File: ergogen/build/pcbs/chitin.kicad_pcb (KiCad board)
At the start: 2 copper layers, 134 x 106.7 mm, 102 parts, among them J1 qwiik_jst

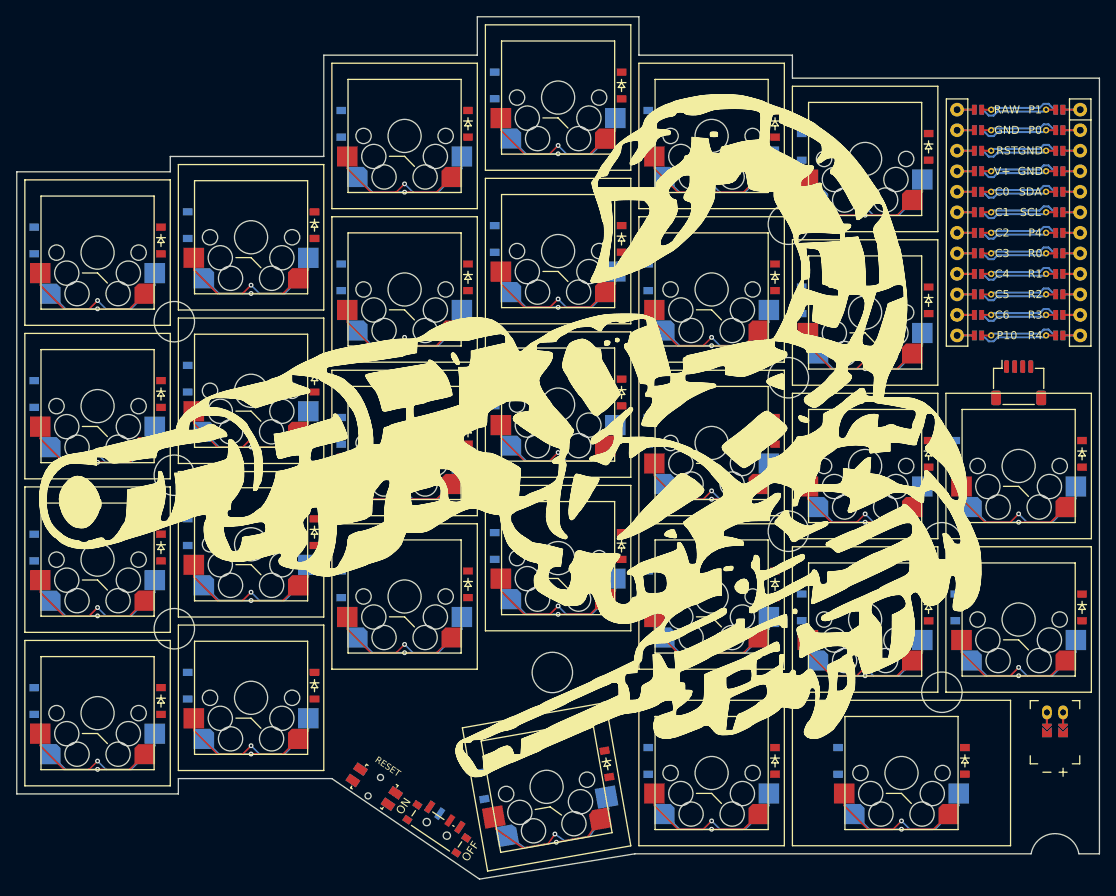
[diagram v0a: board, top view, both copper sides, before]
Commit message: Build
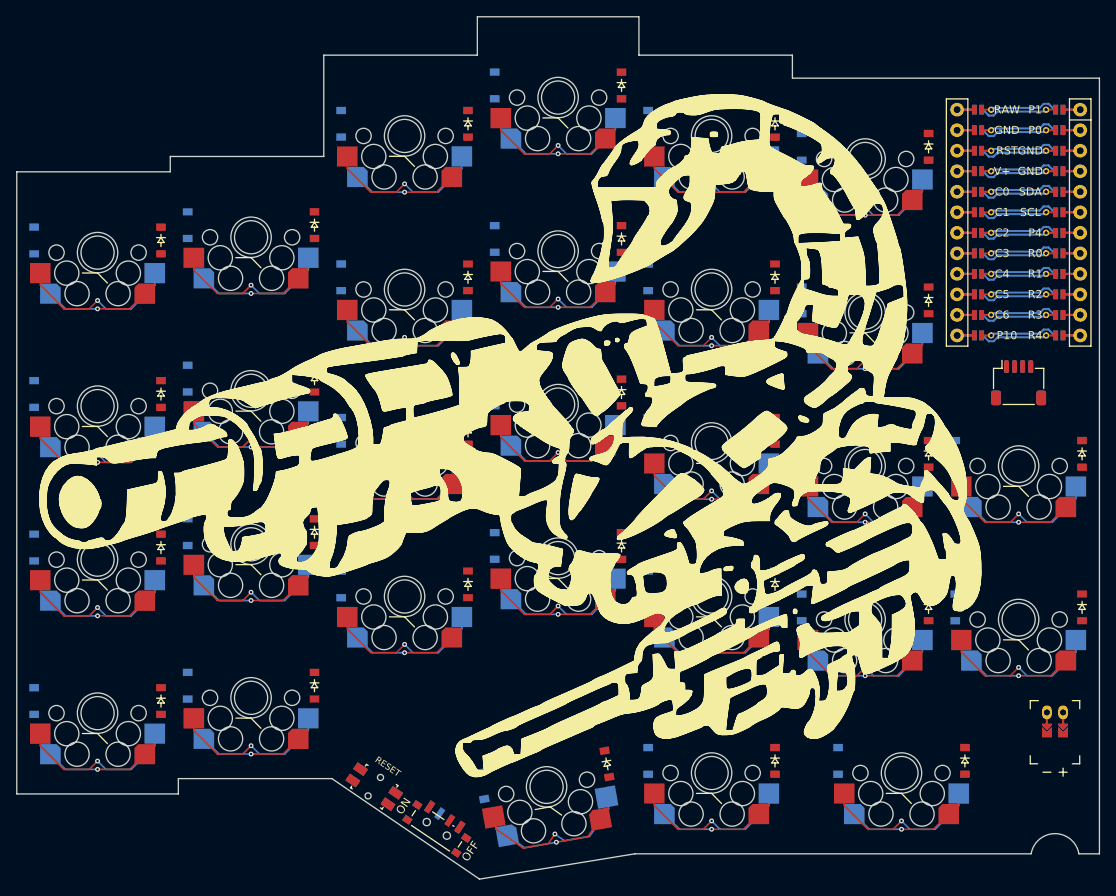
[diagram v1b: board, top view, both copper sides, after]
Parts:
- added MH10: , ceoloide:mounting_hole_npth, F.Cu at (138.0, 116.6)
- added MH11: , ceoloide:mounting_hole_npth, F.Cu at (138.0, 97.6)
- added MH12: , ceoloide:mounting_hole_npth, F.Cu at (138.0, 78.6)
- added MH13: , ceoloide:mounting_hole_npth, F.Cu at (157.0, 130.8)
- added MH14: , ceoloide:mounting_hole_npth, F.Cu at (157.0, 111.8)
- added MH15: , ceoloide:mounting_hole_npth, F.Cu at (157.0, 92.8)
- added MH16: , ceoloide:mounting_hole_npth, F.Cu at (157.0, 73.8)
- added MH17: , ceoloide:mounting_hole_npth, F.Cu at (176.0, 135.6)
- added MH18: , ceoloide:mounting_hole_npth, F.Cu at (176.0, 116.6)
- added MH19: , ceoloide:mounting_hole_npth, F.Cu at (176.0, 97.6)
- added MH20: , ceoloide:mounting_hole_npth, F.Cu at (176.0, 78.6)
- added MH21: , ceoloide:mounting_hole_npth, F.Cu at (195.0, 138.4)
- added MH22: , ceoloide:mounting_hole_npth, F.Cu at (195.0, 119.4)
- added MH23: , ceoloide:mounting_hole_npth, F.Cu at (195.0, 100.4)
- added MH24: , ceoloide:mounting_hole_npth, F.Cu at (195.0, 81.4)
- added MH25: , ceoloide:mounting_hole_npth, F.Cu at (155.6, 159.1)
- added MH26: , ceoloide:mounting_hole_npth, F.Cu at (176.0, 157.4)
- added MH27: , ceoloide:mounting_hole_npth, F.Cu at (199.5, 157.4)
- added MH28: , ceoloide:mounting_hole_npth, F.Cu at (214.0, 138.4)
- added MH29: , ceoloide:mounting_hole_npth, F.Cu at (214.0, 119.4)
- moved MH8 93.5 mm to (119.0, 91.1)
- moved MH5 88.6 mm to (119.0, 148.1)
- moved MH4 76.6 mm to (100.0, 93.0)
- moved MH6 69.6 mm to (119.0, 129.1)
- moved MH7 68.7 mm to (119.0, 110.1)
- moved MH9 67.5 mm to (138.0, 135.6)
- moved MH1 49.4 mm to (100.0, 150.0)
- moved MH3 29.1 mm to (100.0, 112.0)
- moved MH2 14.1 mm to (100.0, 131.0)
